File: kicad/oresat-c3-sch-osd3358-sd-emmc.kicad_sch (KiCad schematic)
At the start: 38 parts, among them J5 DM3BT-DSF-PEJS, Q2 SI7106DN-T1-GE3, U1 OSD3358-512M-BSM, U9 EMMC+RESET+5.1-COMPATIBLE-BA

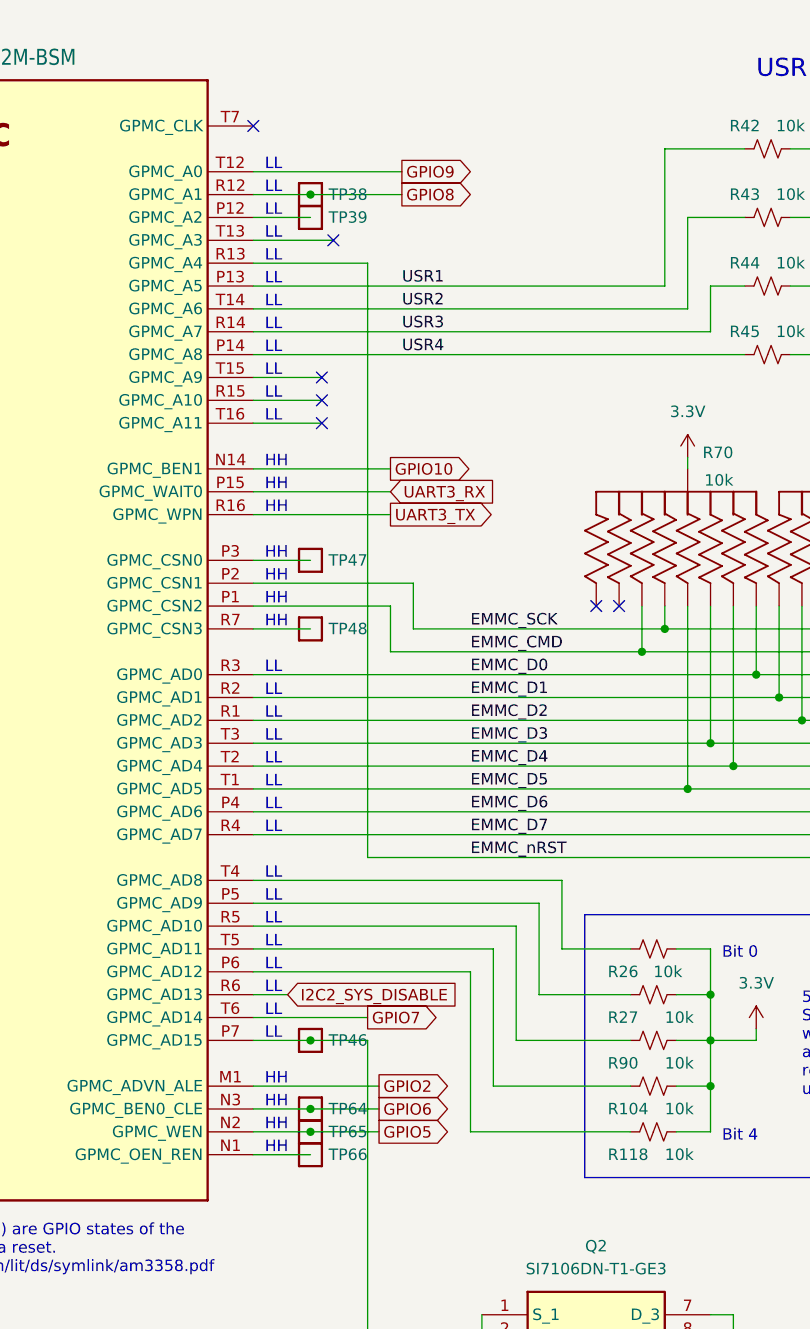
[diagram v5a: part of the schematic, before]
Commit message: Added 2 new GPIO pins
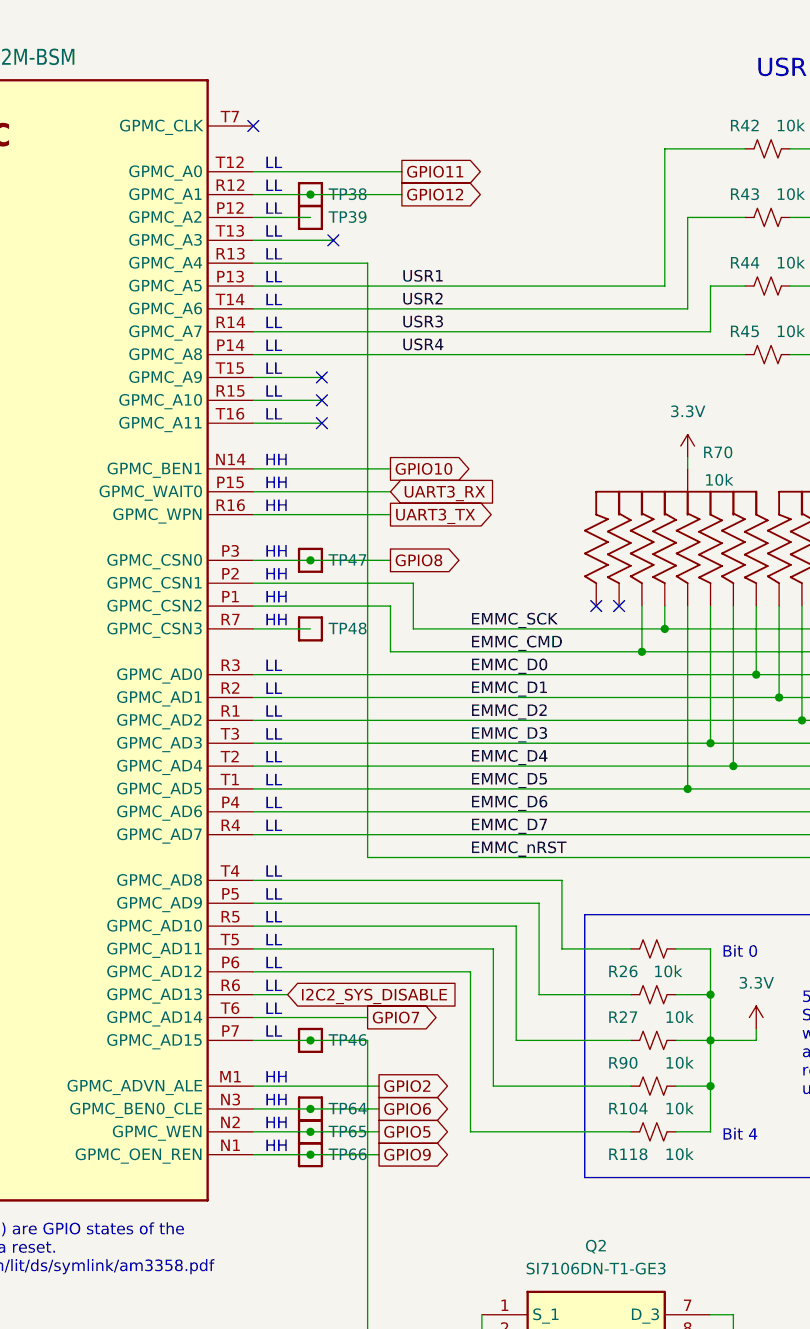
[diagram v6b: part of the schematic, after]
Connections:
- net GPIO8: now also TP47.1, U1.P3 (GPMC_CSN0); no longer TP38.1, U1.R12 (GPMC_A1)
- net GPIO9: now also TP66.1, U1.N1 (GPMC_OEN_REN); no longer U1.T12 (GPMC_A0)
- new net GPIO11: U1.T12 (GPMC_A0)
- new net GPIO12: TP38.1, U1.R12 (GPMC_A1)
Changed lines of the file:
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@@
 	)
 	(junction
+		(at 229.87 215.9)
+		(diameter 0)
+		(color 0 0 0 0)
+	)
+	(junction
 		(at 276.86 243.84)
 		(diameter 0)
@@
 	)
 	(junction
+		(at 229.87 149.86)
+		(diameter 0)
+		(color 0 0 0 0)
+	)
+	(junction
 		(at 300.99 111.76)
 		(diameter 0)
@@
 	(wire
 		(pts
+			(xy 229.87 149.86) (xy 238.76 149.86)
+		)
+		(stroke
+			(width 0)
+			(type default)
+		)
+	)
+	(wire
+		(pts
 			(xy 241.3 152.4) (xy 241.3 157.48)
 		)
@@
 	(wire
 		(pts
+			(xy 229.87 215.9) (xy 237.49 215.9)
+		)
+		(stroke
+			(width 0)
+			(type default)
+		)
+	)
+	(wire
+		(pts
 			(xy 114.3 152.4) (xy 162.56 152.4)
 		)
@@
 		)
 	)
+	(global_label "GPIO9"
+		(shape output)
+		(at 237.49 215.9 0)
+		(fields_autoplaced yes)
+		(effects
+			(font
+				(size 1.27 1.27)
+			)
+			(justify left)
+		)
+		(property "Intersheetrefs" "${INTERSHEET_REFS}"
+			(at 246.16 215.9 0)
+			(effects
+				(font
+					(size 1.27 1.27)
+				)
+				(justify left)
+			)
+		)
+	)
 	(global_label "MRAM_SPI_CLK"
 		(shape output)
@@
 		)
 	)
-	(global_label "GPIO9"
+	(global_label "GPIO11"
 		(shape output)
 		(at 240.03 106.68 0)
@@
 		)
 		(property "Intersheetrefs" "${INTERSHEET_REFS}"
-			(at 248.7 106.68 0)
+			(at 249.9095 106.68 0)
+			(effects
+				(font
+					(size 1.27 1.27)
+				)
+				(justify left)
+			)
+		)
+	)
+	(global_label "GPIO8"
+		(shape output)
+		(at 238.76 149.86 0)
+		(fields_autoplaced yes)
+		(effects
+			(font
+				(size 1.27 1.27)
+			)
+			(justify left)
+		)
+		(property "Intersheetrefs" "${INTERSHEET_REFS}"
+			(at 247.43 149.86 0)
 			(effects
 				(font
@@
 		)
 	)
-	(global_label "GPIO8"
+	(global_label "GPIO12"
 		(shape output)
 		(at 240.03 109.22 0)
@@
 		)
 		(property "Intersheetrefs" "${INTERSHEET_REFS}"
-			(at 248.7 109.22 0)
+			(at 249.9095 109.22 0)
 			(effects
 				(font

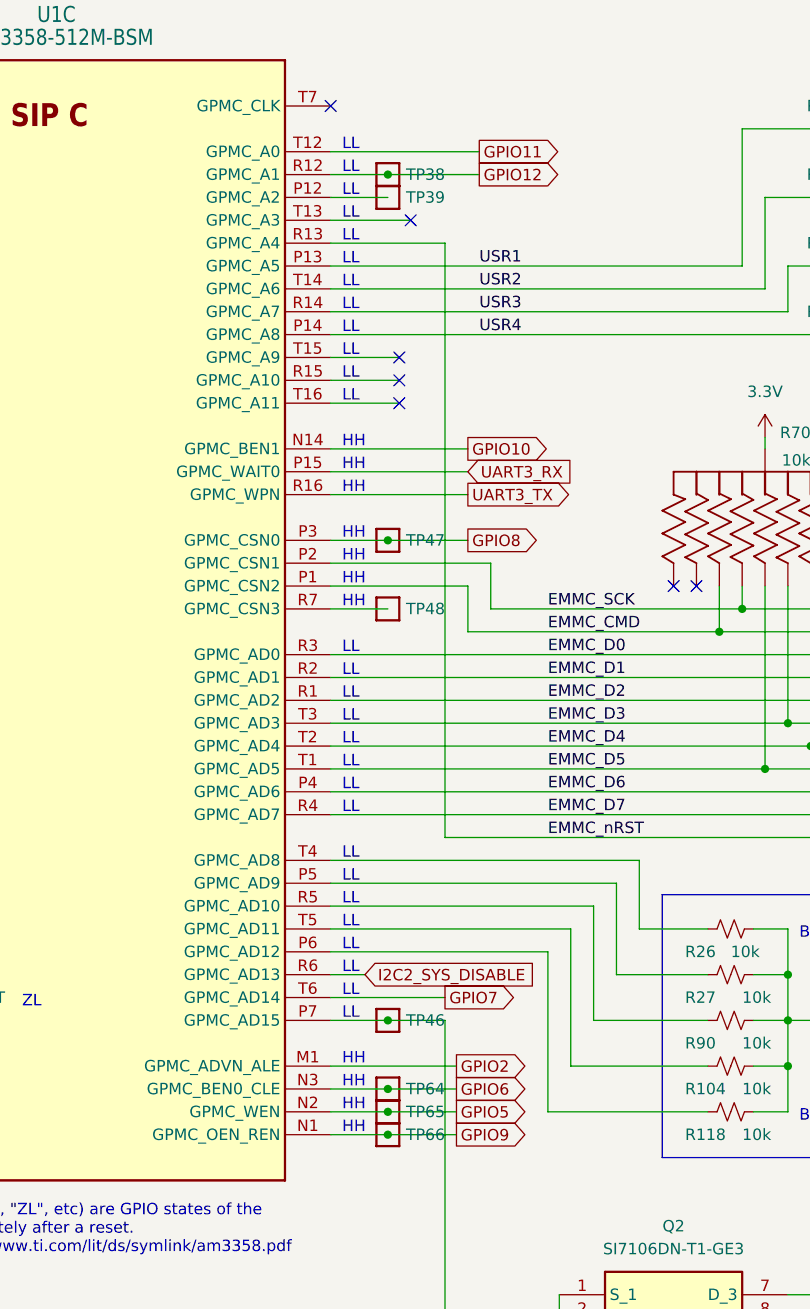
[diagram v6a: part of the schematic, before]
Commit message: - Configured pin headers for UART5 and boot pins to be horizontal - Removed some TPs for GPIO pins
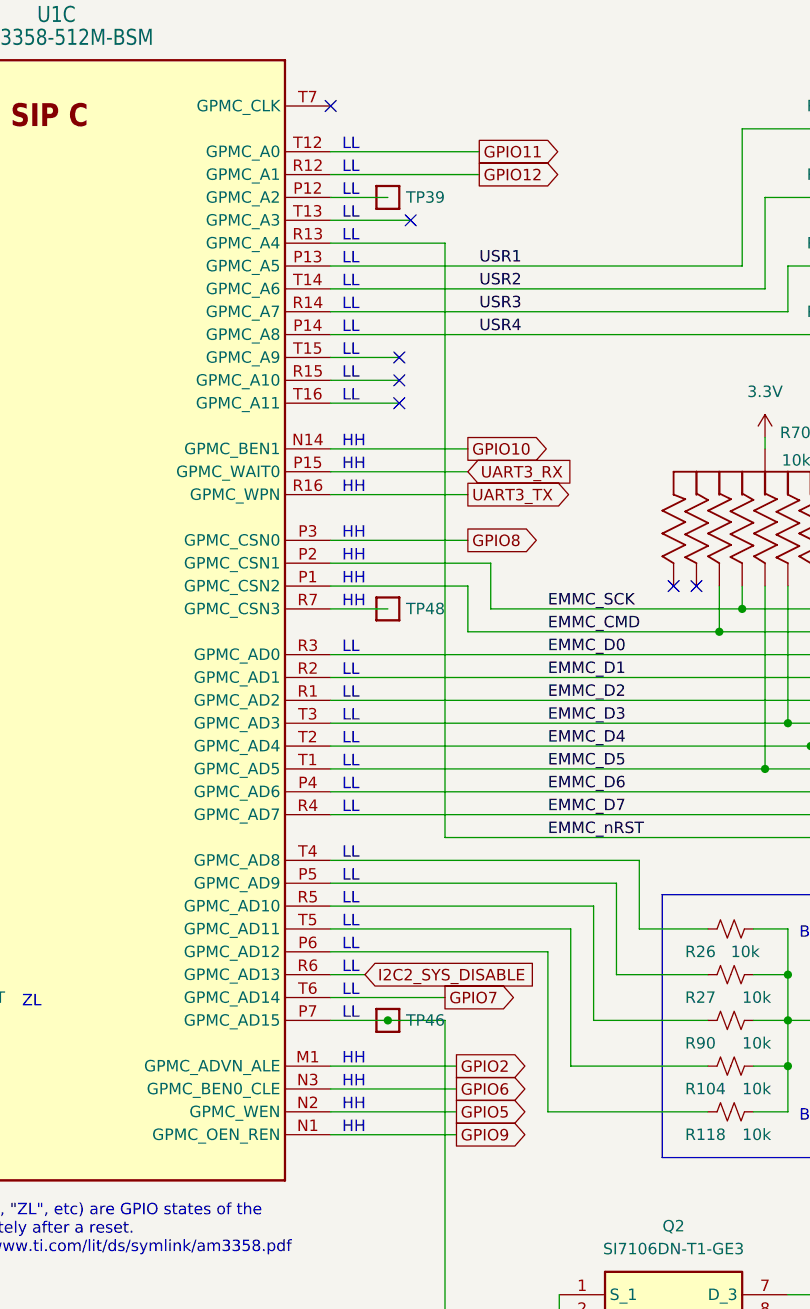
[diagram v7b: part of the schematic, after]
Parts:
- removed TP38, TP47, TP64, TP65, TP66: Test-Point, oresat-misc:TestPoint_Pad_D1.0mm, symbol oresat-misc:Test-Point-1mm-round
